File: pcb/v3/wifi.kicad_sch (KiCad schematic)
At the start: 23 parts, among them U11 TXS0102DCU, U12 TXS0102DCU, U13 CH422E, U8 M8800DU6, U9 ME1502AM5G

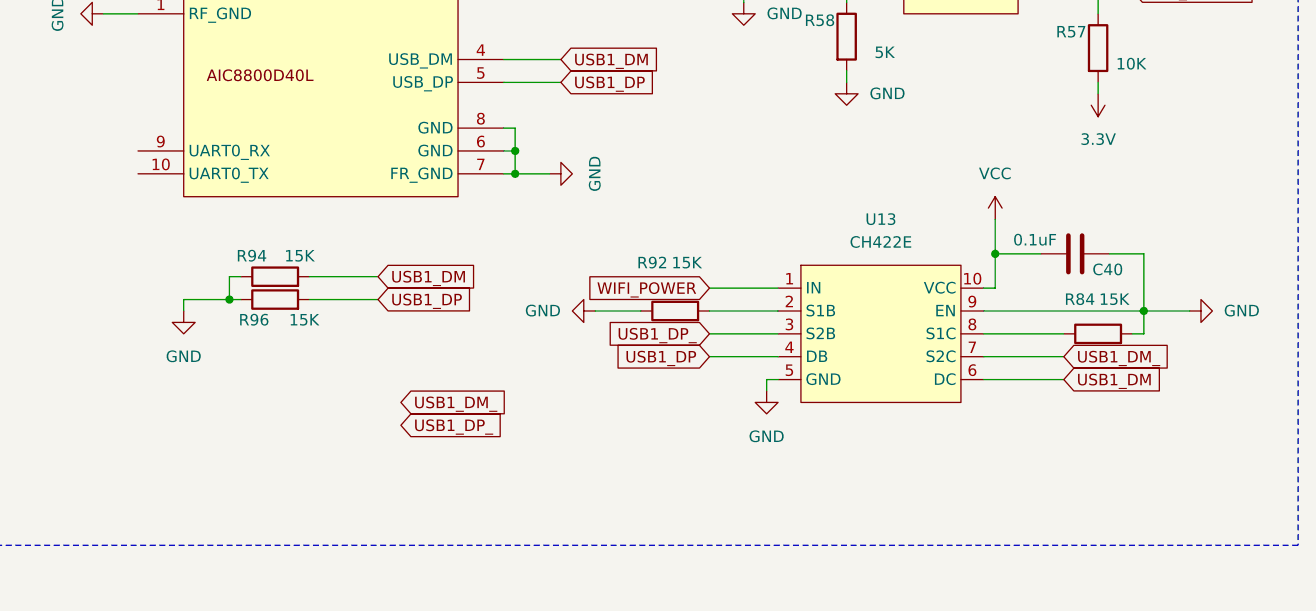
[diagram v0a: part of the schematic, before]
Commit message: up pcb
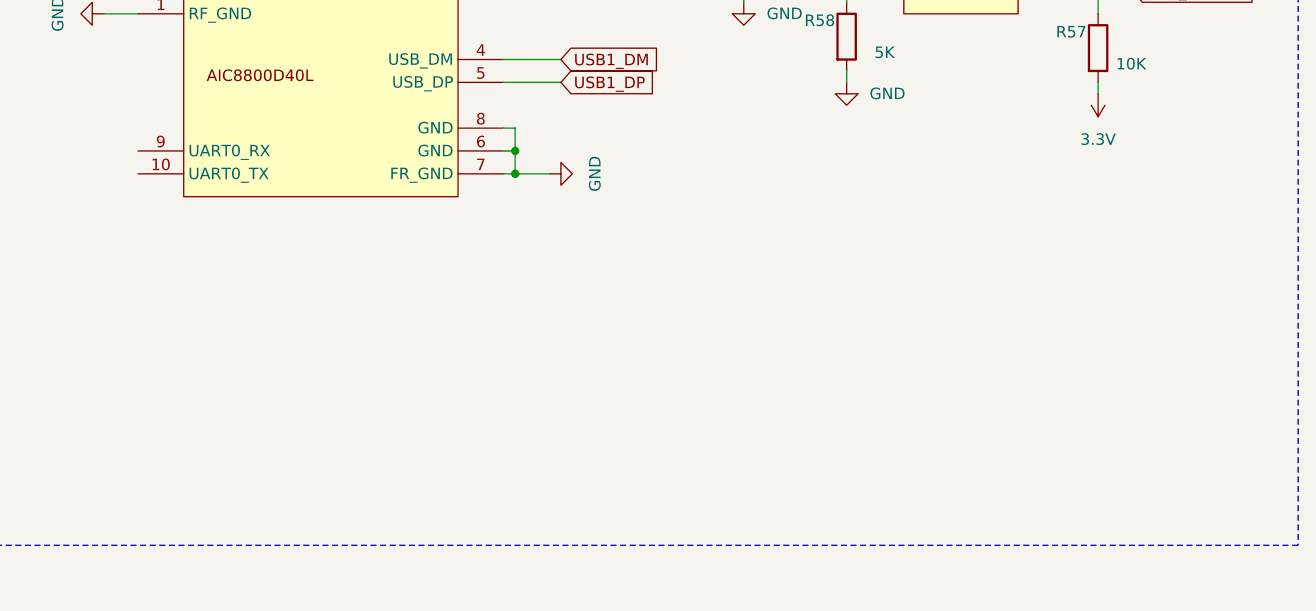
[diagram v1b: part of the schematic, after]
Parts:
- removed C40: 0.1uF, Capacitor_SMD:C_0402_1005Metric_Pad0.74x0.62mm_HandSolder, symbol Device:C
- removed R84, R92: 15K, Resistor_SMD:R_0402_1005Metric_Pad0.72x0.64mm_HandSolder, symbol Device:R
- removed R94, R96: 15K, Capacitor_SMD:C_0402_1005Metric_Pad0.74x0.62mm_HandSolder, symbol Device:R
- removed U13: CH422E, Package_SO:MSOP-10_3x3mm_P0.5mm, symbol coloryr:CH442E
